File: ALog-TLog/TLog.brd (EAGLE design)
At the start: 124.1 x 45.3 mm, 101 parts, among them IC1 ATMEGA644M, J6 5.5x2.1mm Barrel, Q5 MOSFET_PCH-IRLML2244, Q6 MOSFET_PCH-IRLML2244, Q7 MOSFET_PCH-IRLML2244, Q8 MOSFET-NCH-BSS138, Q9 MOSFET-NCH-BSS138, U2 FT231X-Q, U3 915MHz, U4 SX1509, X2 87832-14

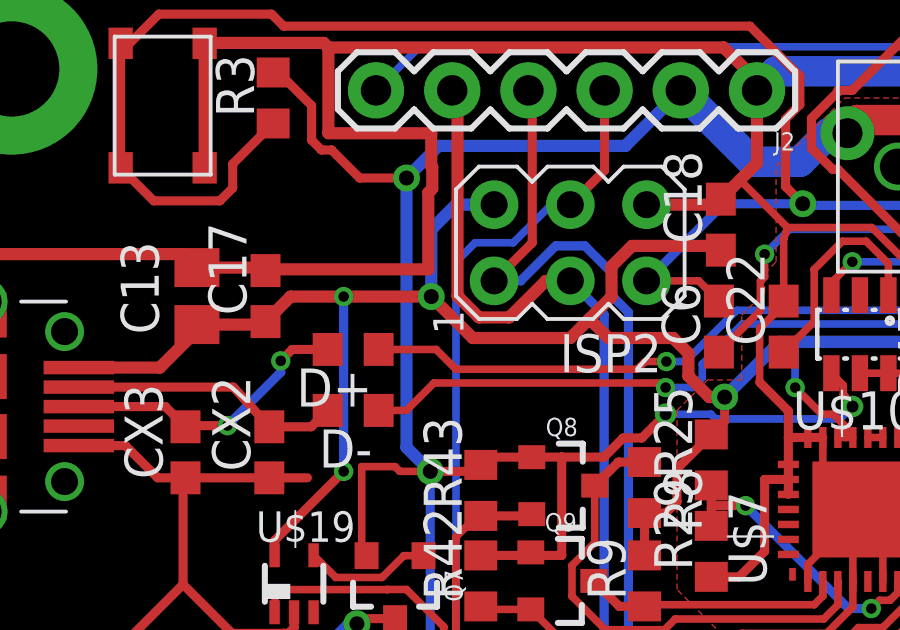
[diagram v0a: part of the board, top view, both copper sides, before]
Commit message: Presumptive Final gerbers for TLog Mrk 1.1
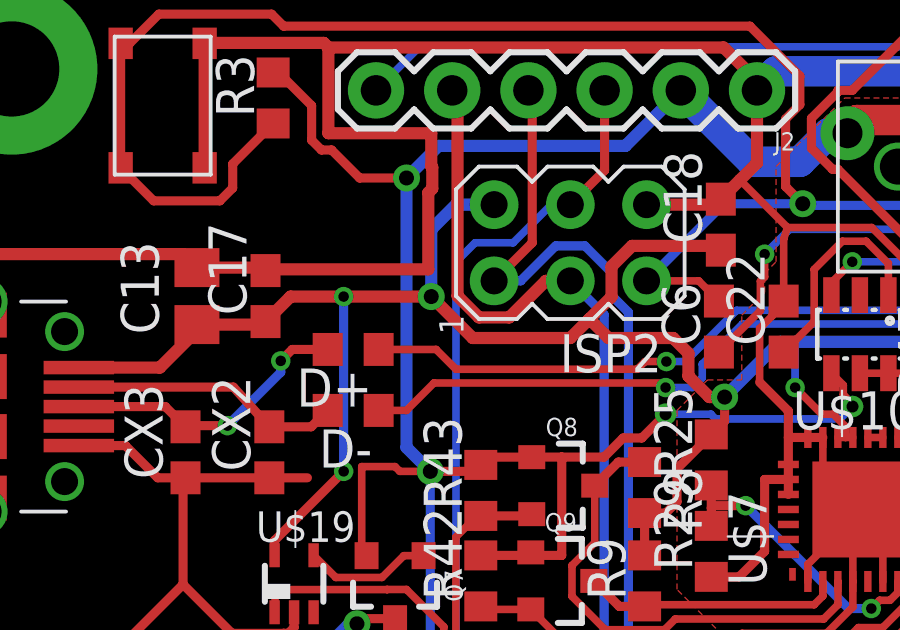
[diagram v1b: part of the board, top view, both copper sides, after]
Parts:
- ISP2: device adafruit:AVRISP -> bschulz:AVRISP
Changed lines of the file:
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@@
 <?xml version="1.0" encoding="utf-8"?>
 <!DOCTYPE eagle SYSTEM "eagle.dtd">
-<eagle version="8.3.2">
+<eagle version="8.5.1">
 <drawing>
 <settings>
@@
 <layer number="22" name="bPlace" color="7" fill="1" visible="yes" active="yes"/>
 <layer number="23" name="tOrigins" color="15" fill="1" visible="yes" active="yes"/>
-<layer number="24" name="bOrigins" color="15" fill="1" visible="yes" active="yes"/>
-<layer number="25" name="tNames" color="7" fill="1" visible="yes" active="yes"/>
-<layer number="26" name="bNames" color="7" fill="1" visible="yes" active="yes"/>
-<layer number="27" name="tValues" color="7" fill="1" visible="yes" active="yes"/>
-<layer number="28" name="bValues" color="7" fill="1" visible="yes" active="yes"/>
+<layer number="24" name="bOrigins" color="15" fill="1" visible="no" active="yes"/>
+<layer number="25" name="tNames" color="7" fill="1" visible="no" active="yes"/>
+<layer number="26" name="bNames" color="7" fill="1" visible="no" active="yes"/>
+<layer number="27" name="tValues" color="7" fill="1" visible="no" active="yes"/>
+<layer number="28" name="bValues" color="7" fill="1" visible="no" active="yes"/>
 <layer number="29" name="tStop" color="7" fill="3" visible="no" active="yes"/>
 <layer number="30" name="bStop" color="7" fill="6" visible="no" active="yes"/>
@@
 <layer number="37" name="tTest" color="7" fill="1" visible="no" active="yes"/>
 <layer number="38" name="bTest" color="7" fill="1" visible="no" active="yes"/>
-<layer number="39" name="tKeepout" color="4" fill="11" visible="yes" active="yes"/>
-<layer number="40" name="bKeepout" color="1" fill="11" visible="yes" active="yes"/>
-<layer number="41" name="tRestrict" color="4" fill="10" visible="yes" active="yes"/>
-<layer number="42" name="bRestrict" color="1" fill="10" visible="yes" active="yes"/>
+<layer number="39" name="tKeepout" color="4" fill="11" visible="no" active="yes"/>
+<layer number="40" name="bKeepout" color="1" fill="11" visible="no" active="yes"/>
+<layer number="41" name="tRestrict" color="4" fill="10" visible="no" active="yes"/>
+<layer number="42" name="bRestrict" color="1" fill="10" visible="no" active="yes"/>
 <layer number="43" name="vRestrict" color="2" fill="10" visible="no" active="yes"/>
 <layer number="44" name="Drills" color="7" fill="1" visible="yes" active="yes"/>
@@
 <wire x1="0.127" y1="45.36525" x2="0.127" y2="0.09525" width="0.254" layer="20"/>
 <rectangle x1="28.477" y1="25.804" x2="28.757" y2="26.254" layer="29"/>
-<text x="4.699" y="39.497" size="1.778" layer="51" font="vector" ratio="10" rot="SR180">RST</text>
-<text x="4.953" y="7.493" size="1.778" layer="51" font="vector" ratio="10" rot="SR180">LOG</text>
+<text x="5.08" y="39.497" size="1.778" layer="51" font="vector" ratio="10" rot="SR180">RST</text>
+<text x="5.08" y="7.747" size="1.778" layer="51" font="vector" ratio="10" rot="SR180">LOG</text>
 <text x="15.60625625" y="8.755959375" size="1.27" layer="51" font="vector" ratio="10" rot="SR180">GND</text>
 <text x="18.377803125" y="9.614803125" size="1.27" layer="51" font="vector" ratio="10" rot="SR225">A0</text>
@@
 parntnership with
 Northern Widget LLC</text>
-<text x="44.7664" y="11.284" size="0.6096" layer="22" rot="MR0">TM</text>
+<text x="43.736" y="10.994" size="0.8128" layer="22" font="vector" ratio="20" rot="MR0" align="bottom-right">TM</text>
 </plain>
 <attributes>
@@
 <param name="dpMaxLengthDifference" value="10mm"/>
 <param name="dpGapFactor" value="2.5"/>
-<param name="checkGrid" value="0"/>
 <param name="checkAngle" value="0"/>
 <param name="checkFont" value="1"/>
 <param name="checkRestrict" value="1"/>
+<param name="checkStop" value="0"/>
+<param name="checkValues" value="0"/>
 <param name="useDiameter" value="13"/>
 <param name="maxErrors" value="50"/>
@@
 <attribute name="MPN" value="MF-NSMF020-2" x="79.8195" y="22.352" size="1.778" layer="27" rot="R180" display="off"/>
 </element>
-<element name="ISP2" library="adafruit" library_urn="urn:adsk.eagle:library:420" package="AVRISP" value="AVRISP-6" x="21.209" y="37.084" smashed="yes" rot="R90">
+<element name="ISP2" library="bschulz" package="AVRISP" value="AVRISP-6" x="21.209" y="37.084" smashed="yes" rot="R90">
 <attribute name="DIGIKEY" value="609-3234-ND" x="21.209" y="37.084" size="1.778" layer="27" rot="R90" display="off"/>
 <attribute name="MF" value="Amphenol" x="21.209" y="37.084" size="1.778" layer="27" rot="R90" display="off"/>
